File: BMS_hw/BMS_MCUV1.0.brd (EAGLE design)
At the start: 60 x 30 mm, 48 parts, among them IC2 SST25VF020B804ISA, J1 22-27-2051-05, J2 22-27-2051-05, J3 22-27-2041-04, J4 22-27-2051-05, Q2 32.768kHz, U1 NCP1117LP-PG, X1 87758-2016

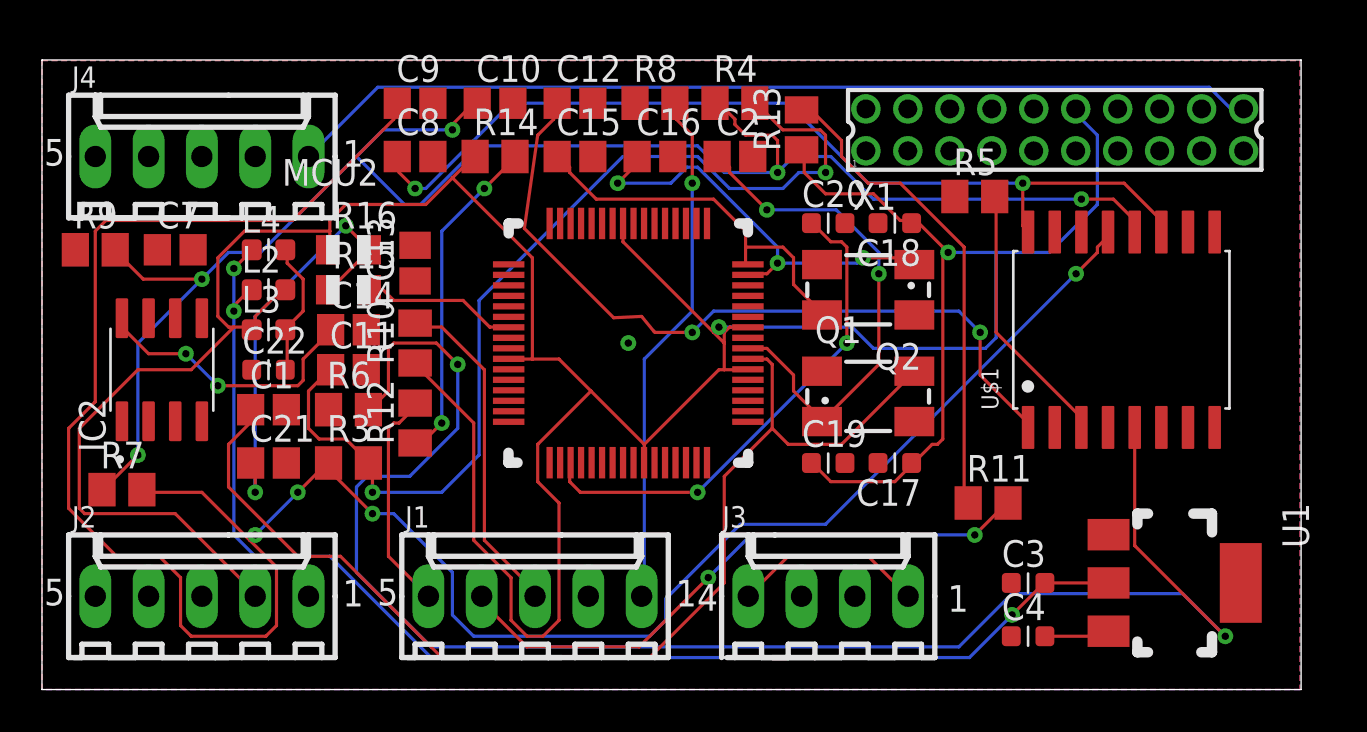
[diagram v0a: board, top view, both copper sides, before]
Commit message: erroe removed
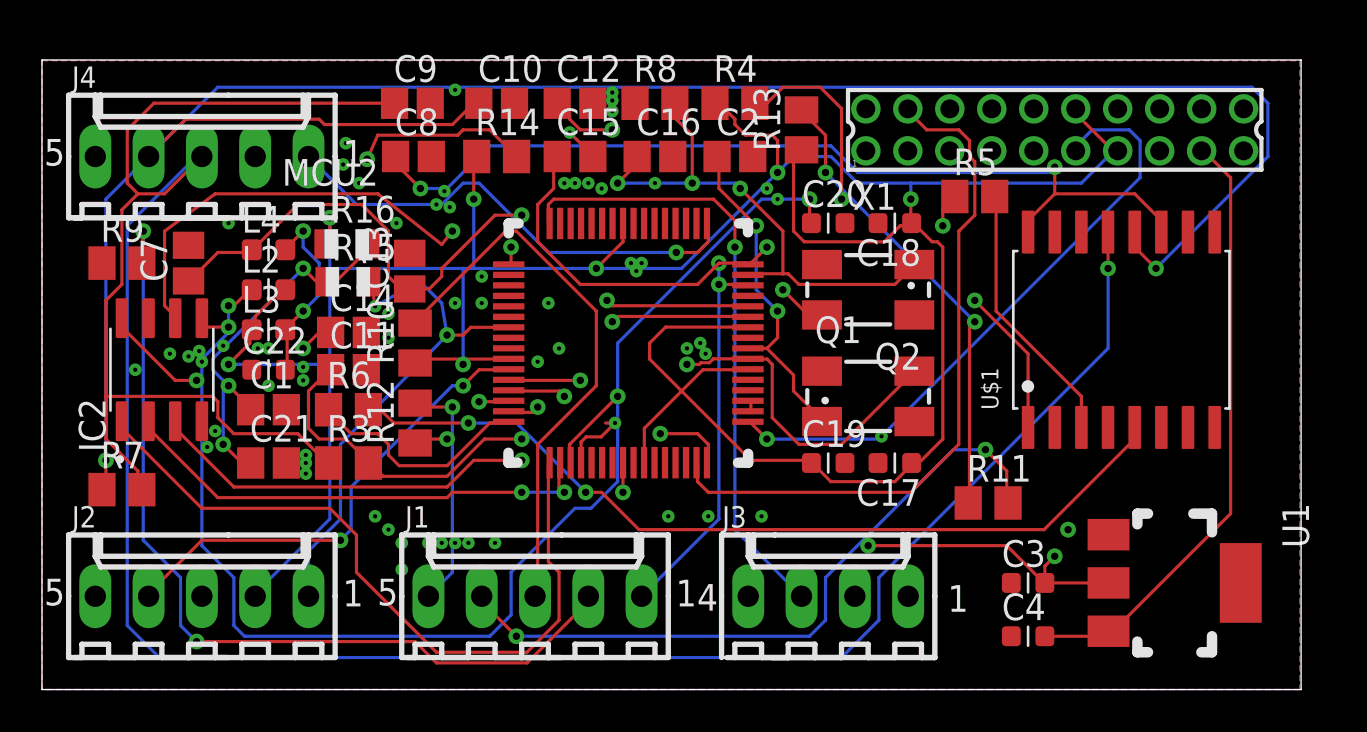
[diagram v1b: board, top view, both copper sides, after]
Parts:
- moved R9 1.42 mm to (3.81, 20.3)
- moved C7 0.90 mm to (6.99, 20.3), turned to 90 degrees
- moved C13 0.46 mm to (17.5, 19.9)
- moved R15 0.38 mm to (14.6, 19.4)
- moved R16 0.29 mm to (14.5, 21.2)
- moved C9 0.13 mm to (17.7, 27.9)
- moved C14 0.13 mm to (14.6, 17.0)
- moved C10 0.08 mm to (21.7, 27.9)
- moved C8 0.08 mm to (17.7, 25.4)
- moved R14 0.08 mm to (21.7, 25.4)
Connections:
- net DGND renamed VSS
- removed net 12V_AUX: X1.17
- removed net DC_1: C13.1
- removed net GO_03: X1.5
- removed net GO_04: X1.15
- removed net HOLD#: IC2.7
- removed net ICSP_!MCLR!_VPP_TARGET: MCU2.7, R15.2
- removed net ISM: X1.1
- removed net KEY: X1.10
- removed net N$5: C4.2, U1.3
- removed net RX_O: X1.16
- removed net SCL_O: X1.3
- removed net SDA_O: X1.13
- removed net SYS_VOLT: X1.8
- removed net SYS_VOLT_SEL: X1.18
- removed net TX_0: X1.6
- removed net T_SUPPLY: J3.1, J3.4
- removed net UC3: C7.1
- removed net VUSB3V3: MCU2.35
- new net 15V_AUX: C4.2, U1.3, X1.17
- new net DBG_RX: J3.3, MCU2.64
- new net DBG_TX: J3.2, MCU2.12
- new net FAULT: MCU2.13, X1.5
- new net N$40: MCU2.29
- new net N$41: MCU2.30
- new net N$42: MCU2.58
- new net N$43: MCU2.59
- new net N$44: MCU2.4
- new net N$45: MCU2.5
- new net N$46: MCU2.6
- new net N$47: MCU2.8
- new net N$66: MCU2.60
- new net N$67: MCU2.61
- new net N$68: MCU2.62
- new net N$69: MCU2.63
- new net N$70: MCU2.3
- new net N$71: MCU2.21
- new net N$72: MCU2.22
- new net N$73: MCU2.23
- new net N$74: MCU2.50
- new net N$75: MCU2.51
- new net N$76: MCU2.52
- new net N$77: MCU2.55
- new net N$78: MCU2.45
- new net N$79: MCU2.36
- new net N$80: MCU2.37
- new net N$81: MCU2.2
- new net N$82: MCU2.34, MCU2.35
- new net PCHG_FET: MCU2.31, X1.4
- net !MCLR: now also MCU2.7, R15.2
- net 3.3V: now also C13.1, C7.1
- net CANH: now also C9.1, R3.1, R7.2, U$1.13; no longer X1.14
- net CANL: now also C10.1, R4.1, R7.1, U$1.12; no longer X1.4
- net CAN_RX: now also MCU2.15
- net CAN_TX: now also MCU2.16
- net CE#: now also MCU2.17
- net C_FET: now also MCU2.14
- net D_FET: now also MCU2.1
- net GND: now also IC2.7, J3.1, J3.4, X1.1, X1.10, X1.14, X1.15, X1.16, X1.18, X1.20, X1.3, X1.6, X1.8
- net ICSPCLK: now also MCU2.24
- net ICSPDAT: now also MCU2.11
- net INTL_IN2: now also MCU2.46
- net INTL_OUT: now also MCU2.49; no longer X1.20
- net ISP: now also MCU2.33
- net N$10: now also MCU2.54; no longer C10.1, R4.1, R7.1, U$1.12
- net N$29: now also MCU2.27; no longer J3.2
- net N$30: now also MCU2.28; no longer J3.3
- net N$9: now also MCU2.53; no longer C9.1, R3.1, R7.2, U$1.13
- net SCK: now also MCU2.44
- net SI: now also MCU2.43
- net SO: now also MCU2.18
- net VDD: now also X1.13
- net WP#: now also MCU2.32
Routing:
- net N$9: track 111.8 -> 0.00 mm, vias 4 -> 0
- net CANL: track 38.0 -> 137.6 mm, vias 0 -> 3
- net CANH: track 45.4 -> 132.3 mm, vias 0 -> 1
- net N$10: track 76.0 -> 0.00 mm, vias 4 -> 0
- net CAN_RX: track 0.00 -> 44.8 mm, vias 0 -> 2
- net D_FET: track 0.00 -> 41.6 mm, vias 0 -> 1
- net N$6: track 76.8 -> 41.2 mm
- net C_FET: track 0.00 -> 35.5 mm, vias 0 -> 1
- net SCK: track 0.00 -> 35.4 mm, vias 0 -> 2
- net CE#: track 0.00 -> 35.0 mm
- net PCHG_FET: track 0.00 -> 33.0 mm
- net ISP: track 0.00 -> 29.8 mm, vias 0 -> 1
- net DBG_RX: track 0.00 -> 29.6 mm, vias 0 -> 1
- net ICSPCLK: track 0.00 -> 29.3 mm, vias 0 -> 1
- net 15V_AUX: track 0.00 -> 29.3 mm
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- added copper zone on layer 16, net GND
- removed copper zone on layer 16, net 3.3V
